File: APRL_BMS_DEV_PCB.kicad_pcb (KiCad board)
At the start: 4 copper layers, 2 parts, among them U1 BQ756506-Q1, U2 STM32F446RCTx

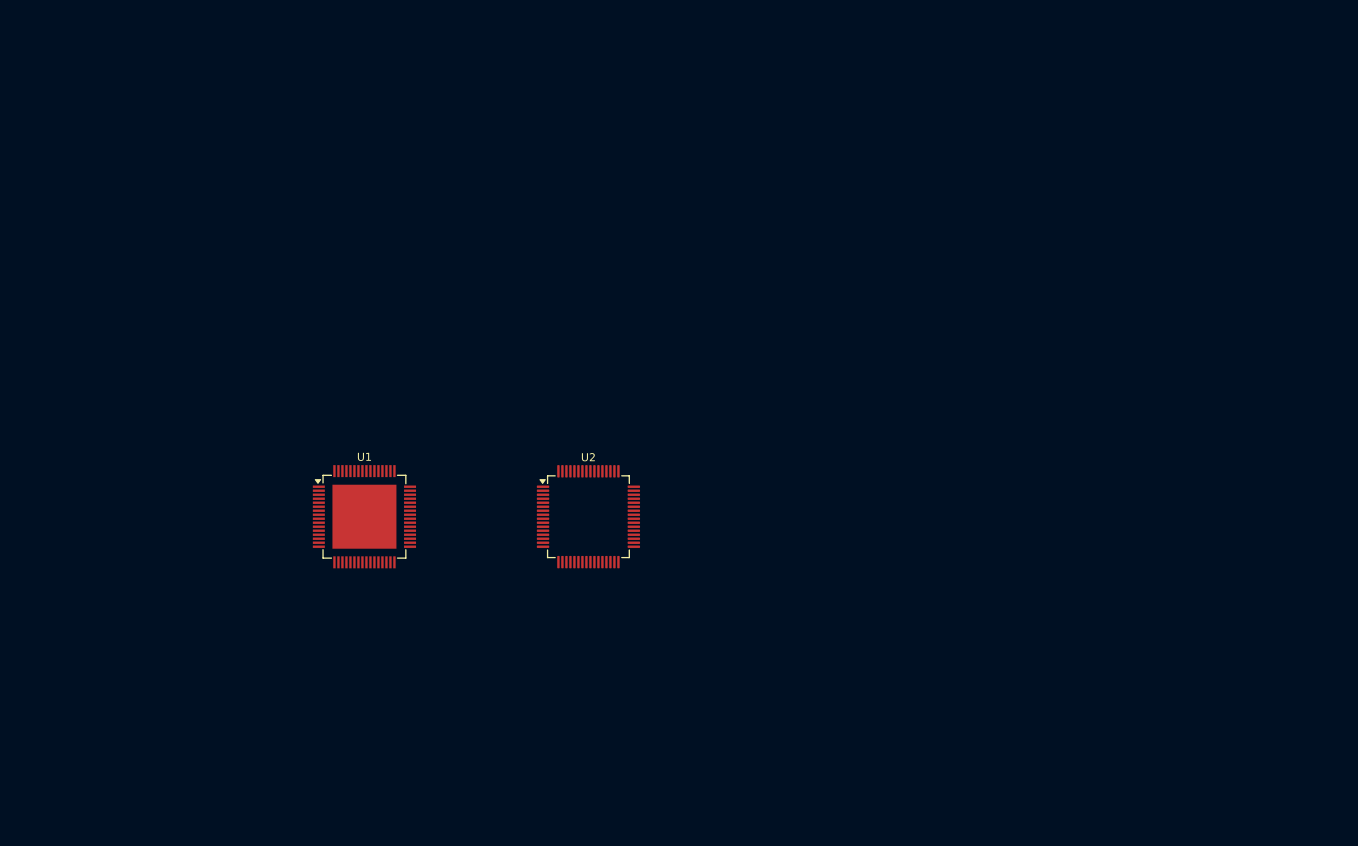
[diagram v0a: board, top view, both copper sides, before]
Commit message: Edited PCB a little
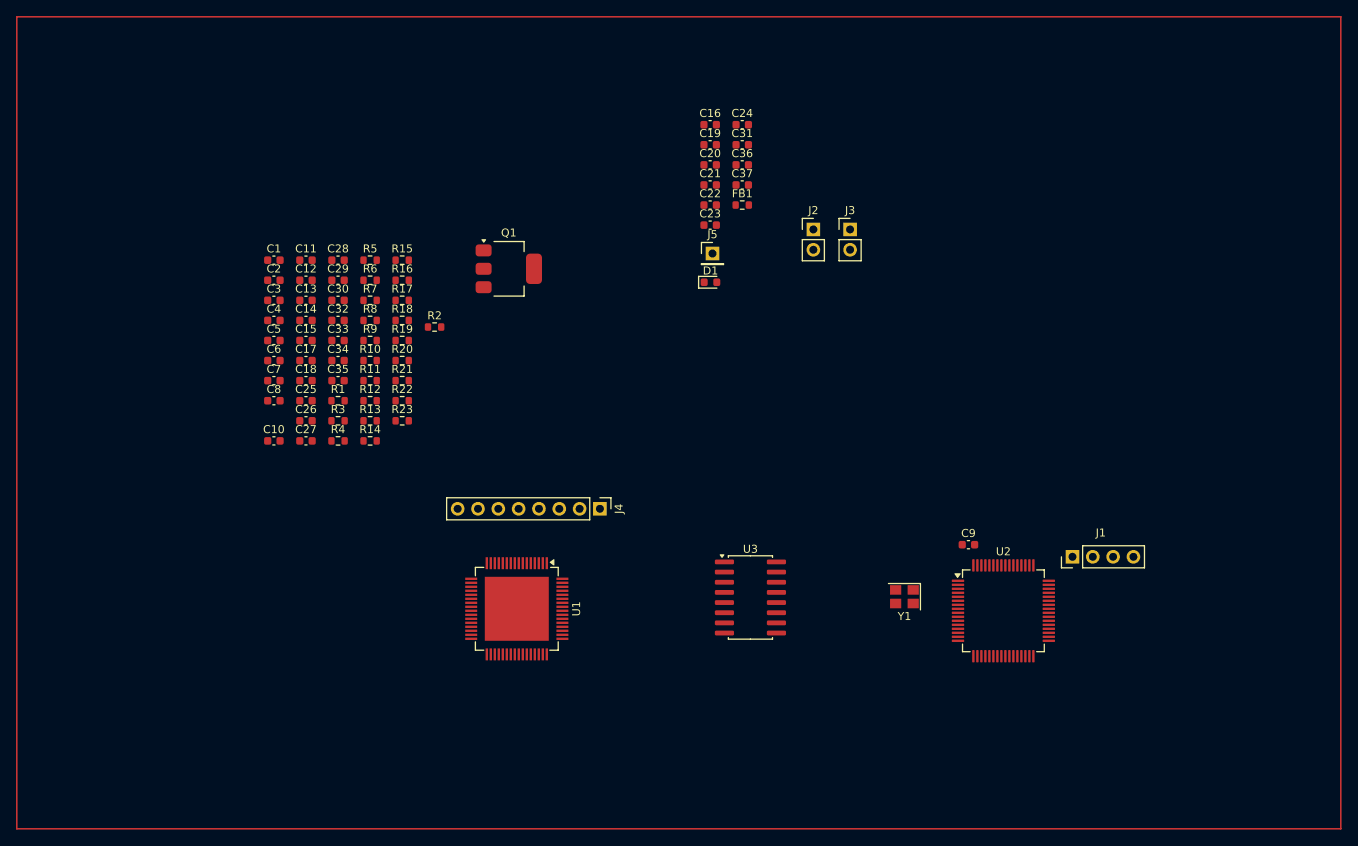
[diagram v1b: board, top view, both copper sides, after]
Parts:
- added C1: 1u, Capacitor_SMD:C_0603_1608Metric, F.Cu at (80.2, 61.4)
- added C10: 10n, Capacitor_SMD:C_0603_1608Metric, F.Cu at (80.2, 84.0)
- added C11: 1u, Capacitor_SMD:C_0603_1608Metric, F.Cu at (84.2, 61.4)
- added C12: 4.7u, Capacitor_SMD:C_0603_1608Metric, F.Cu at (84.2, 63.9)
- added C13: 20n, Capacitor_SMD:C_0603_1608Metric, F.Cu at (84.2, 66.5)
- added C14: .47u, Capacitor_SMD:C_0603_1608Metric, F.Cu at (84.2, 69.0)
- added C15: 0.1u, Capacitor_SMD:C_0603_1608Metric, F.Cu at (84.2, 71.5)
- added C16: 0.2u, Capacitor_SMD:C_0603_1608Metric, F.Cu at (134.7, 44.5)
- added C17: .56u, Capacitor_SMD:C_0603_1608Metric, F.Cu at (84.2, 74.0)
- added C18: 10u, Capacitor_SMD:C_0603_1608Metric, F.Cu at (84.2, 76.5)
- added C19: 1.5u, Capacitor_SMD:C_0603_1608Metric, F.Cu at (134.7, 47.0)
- added C2: 100n, Capacitor_SMD:C_0603_1608Metric, F.Cu at (80.2, 63.9)
- added C20: 1.5u, Capacitor_SMD:C_0603_1608Metric, F.Cu at (134.7, 49.5)
- added C21: 1.5u, Capacitor_SMD:C_0603_1608Metric, F.Cu at (134.7, 52.0)
- added C22: 1.5u, Capacitor_SMD:C_0603_1608Metric, F.Cu at (134.7, 54.5)
- added C23: 1.5u, Capacitor_SMD:C_0603_1608Metric, F.Cu at (134.7, 57.0)
- added C24: 1.5u, Capacitor_SMD:C_0603_1608Metric, F.Cu at (138.7, 44.5)
- added C25: 1.5u, Capacitor_SMD:C_0603_1608Metric, F.Cu at (84.2, 79.0)
- added C26: 1.5u, Capacitor_SMD:C_0603_1608Metric, F.Cu at (84.2, 81.5)
- added C27: 1.5u, Capacitor_SMD:C_0603_1608Metric, F.Cu at (84.2, 84.0)
- added C28: 1.5u, Capacitor_SMD:C_0603_1608Metric, F.Cu at (88.2, 61.4)
- added C29: 1.5u, Capacitor_SMD:C_0603_1608Metric, F.Cu at (88.2, 63.9)
- added C3: 30p, Capacitor_SMD:C_0603_1608Metric, F.Cu at (80.2, 66.5)
- added C30: 1.5u, Capacitor_SMD:C_0603_1608Metric, F.Cu at (88.2, 66.5)
- added C31: 1.5u, Capacitor_SMD:C_0603_1608Metric, F.Cu at (138.7, 47.0)
- added C32: 1.5u, Capacitor_SMD:C_0603_1608Metric, F.Cu at (88.2, 69.0)
- added C33: 2.2u, Capacitor_SMD:C_0603_1608Metric, F.Cu at (88.2, 71.5)
- added C34: 2.2u, Capacitor_SMD:C_0603_1608Metric, F.Cu at (88.2, 74.0)
- added C35: 1u, Capacitor_SMD:C_0603_1608Metric, F.Cu at (88.2, 76.5)
- added C36: 0.1u, Capacitor_SMD:C_0603_1608Metric, F.Cu at (138.7, 49.5)
- added C37: 0.1u, Capacitor_SMD:C_0603_1608Metric, F.Cu at (138.7, 52.0)
- added C4: 30p, Capacitor_SMD:C_0603_1608Metric, F.Cu at (80.2, 69.0)
- added C5: 10u, Capacitor_SMD:C_0603_1608Metric, F.Cu at (80.2, 71.5)
- added C6: 100n, Capacitor_SMD:C_0603_1608Metric, F.Cu at (80.2, 74.0)
- added C7: 100n, Capacitor_SMD:C_0603_1608Metric, F.Cu at (80.2, 76.5)
- added C8: 100n, Capacitor_SMD:C_0603_1608Metric, F.Cu at (80.2, 79.0)
- added C9: 100n, Capacitor_SMD:C_0603_1608Metric, F.Cu at (167.0, 97.0)
- added D1: RED, LED_SMD:LED_0603_1608Metric, F.Cu at (134.8, 64.2)
- added FB1: 120R, Resistor_SMD:R_0603_1608Metric, F.Cu at (138.7, 54.5)
- added J1: Conn_01x04_Pin, Connector_PinHeader_2.54mm:PinHeader_1x04_P2.54mm_Vertical, F.Cu at (180.0, 98.5)
- added J2: Conn_01x02_Pin, Connector_PinHeader_2.54mm:PinHeader_1x02_P2.54mm_Vertical, F.Cu at (147.6, 57.6)
- added J3: Conn_01x02_Pin, Connector_PinHeader_2.54mm:PinHeader_1x02_P2.54mm_Vertical, F.Cu at (152.2, 57.6)
- added J4: Conn_01x08_Pin, Connector_PinHeader_2.54mm:PinHeader_1x08_P2.54mm_Vertical, F.Cu at (120.9, 92.5)
- added J5: Conn_01x01_Pin, Connector_PinHeader_2.54mm:PinHeader_1x01_P2.54mm_Vertical, F.Cu at (135.0, 60.6)
- added Q1: Q_NPN, Package_TO_SOT_SMD:SOT-223, F.Cu at (109.5, 62.5)
- added R1: 10K, Resistor_SMD:R_0603_1608Metric, F.Cu at (88.2, 79.0)
- added R10: 100, Resistor_SMD:R_0603_1608Metric, F.Cu at (92.2, 74.0)
- added R11: 100, Resistor_SMD:R_0603_1608Metric, F.Cu at (92.2, 76.5)
- added R12: 100, Resistor_SMD:R_0603_1608Metric, F.Cu at (92.2, 79.0)
- added R13: 100, Resistor_SMD:R_0603_1608Metric, F.Cu at (92.2, 81.5)
- added R14: 100, Resistor_SMD:R_0603_1608Metric, F.Cu at (92.2, 84.0)
- added R15: 6.2, Resistor_SMD:R_0603_1608Metric, F.Cu at (96.2, 61.4)
- added R16: 100, Resistor_SMD:R_0603_1608Metric, F.Cu at (96.2, 63.9)
- added R17: 30, Resistor_SMD:R_0603_1608Metric, F.Cu at (96.2, 66.5)
- added R18: 400, Resistor_SMD:R_0603_1608Metric, F.Cu at (96.2, 69.0)
- added R19: 500, Resistor_SMD:R_0603_1608Metric, F.Cu at (96.2, 71.5)
- added R2: 1.2K, Resistor_SMD:R_0603_1608Metric, F.Cu at (100.3, 69.8)
- added R20: 10, Resistor_SMD:R_0603_1608Metric, F.Cu at (96.2, 74.0)
- added R21: 100k, Resistor_SMD:R_0603_1608Metric, F.Cu at (96.2, 76.5)
- added R22: 100k, Resistor_SMD:R_0603_1608Metric, F.Cu at (96.2, 79.0)
- added R23: 4.7k, Resistor_SMD:R_0603_1608Metric, F.Cu at (96.2, 81.5)
- added R3: 6.2, Resistor_SMD:R_0603_1608Metric, F.Cu at (88.2, 81.5)
- added R4: 6.2, Resistor_SMD:R_0603_1608Metric, F.Cu at (88.2, 84.0)
- added R5: 6.2, Resistor_SMD:R_0603_1608Metric, F.Cu at (92.2, 61.4)
- added R6: 6.2, Resistor_SMD:R_0603_1608Metric, F.Cu at (92.2, 63.9)
- added R7: 6.2, Resistor_SMD:R_0603_1608Metric, F.Cu at (92.2, 66.5)
- added R8: 6.2, Resistor_SMD:R_0603_1608Metric, F.Cu at (92.2, 69.0)
- added R9: 100, Resistor_SMD:R_0603_1608Metric, F.Cu at (92.2, 71.5)
- added U3: ISO7741DWR, Package_SO:SOIC-16W_5.3x10.2mm_P1.27mm, F.Cu at (139.8, 103.6)
- added Y1: 20MHz, Crystal:Crystal_SMD_3225-4Pin_3.2x2.5mm, F.Cu at (159.0, 103.5)
- moved U2 53.2 mm to (171.4, 105.3)
- moved U1 22.3 mm to (110.5, 105.0), turned to -90 degrees
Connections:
- U1 pad 1: unconnected-(U1-BAT-Pad1) -> /BAT
- U1 pad 22: unconnected-(U1-CB6-Pad22) -> /CB6
- U1 pad 23: unconnected-(U1-VC6-Pad23) -> /VC6
- U1 pad 24: unconnected-(U1-CB5-Pad24) -> /CB5
- U1 pad 25: unconnected-(U1-VC5-Pad25) -> /VC5
- U1 pad 26: unconnected-(U1-CB4-Pad26) -> /CB4
- U1 pad 27: unconnected-(U1-VC4-Pad27) -> /VC4
- U1 pad 28: unconnected-(U1-CB3-Pad28) -> /CB3
- U1 pad 29: unconnected-(U1-VC3-Pad29) -> /VC3
- U1 pad 30: unconnected-(U1-CB2-Pad30) -> /CB2
- U1 pad 31: unconnected-(U1-VC2-Pad31) -> /VC2
- U1 pad 32: unconnected-(U1-CB1-Pad32) -> /CB1
- U1 pad 33: unconnected-(U1-VC1-Pad33) -> /VC1
- U1 pad 34: unconnected-(U1-CB0-Pad34) -> /CB0
- U1 pad 35: unconnected-(U1-VC0-Pad35) -> /VC0
- U1 pad 37: unconnected-(U1-REFHP-Pad37) -> /REFHP
- U1 pad 38: unconnected-(U1-AVDD-Pad38) -> /AVDD
- U1 pad 44: unconnected-(U1-NEG5V-Pad44) -> Net-(U1-NEG5V)
- U1 pad 45: unconnected-(U1-CVDD-Pad45) -> /CVDD
- U1 pad 47: unconnected-(U1-LDOIN-Pad47) -> /LDOIN
- U1 pad 48: unconnected-(U1-NPNB-Pad48) -> /NPNB
- U1 pad 49: unconnected-(U1-DVDD-Pad49) -> /DVDD
- U1 pad 51: unconnected-(U1-TSREF-Pad51) -> Net-(J5-Pin_1)
- U1 pad 52: unconnected-(U1-RX-Pad52) -> /RX_BMS
- U1 pad 53: unconnected-(U1-TX-Pad53) -> /TX_BMS
- U1 pad 54: unconnected-(U1-GPIO8-Pad54) -> /GPIO1
- U1 pad 55: unconnected-(U1-GPIO7-Pad55) -> /GPIO2
- U1 pad 56: unconnected-(U1-GPIO6-Pad56) -> /GPIO3
- U1 pad 57: unconnected-(U1-GPIO5-Pad57) -> /GPIO4
- U1 pad 58: unconnected-(U1-GPIO4-Pad58) -> /GPIO5
- U1 pad 59: unconnected-(U1-GPIO3-Pad59) -> /GPIO6
- U1 pad 60: unconnected-(U1-GPIO2-Pad60) -> /GPIO7
- U1 pad 61: unconnected-(U1-GPIO1-Pad61) -> /GPIO8
- U1 pad 62: unconnected-(U1-NFAULT-Pad62) -> /NFAULT
- U1 pad 63: unconnected-(U1-SRN-Pad63) -> GND
- U1 pad 64: unconnected-(U1-SRP-Pad64) -> /CELL_0
- U2 pad 30: unconnected-(U2-VCAP_1-Pad30) -> Net-(U2-VCAP_1)
- U2 pad 39: unconnected-(U2-PC8-Pad39) -> /NFAULT_IN
- U2 pad 5: Net-(U2-PH0) -> /OSC_IN
- U2 pad 6: Net-(U2-PH1) -> /OSC_OUT
